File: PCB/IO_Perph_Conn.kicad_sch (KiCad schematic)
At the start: 7 parts, among them U2 STM32MP157FABx

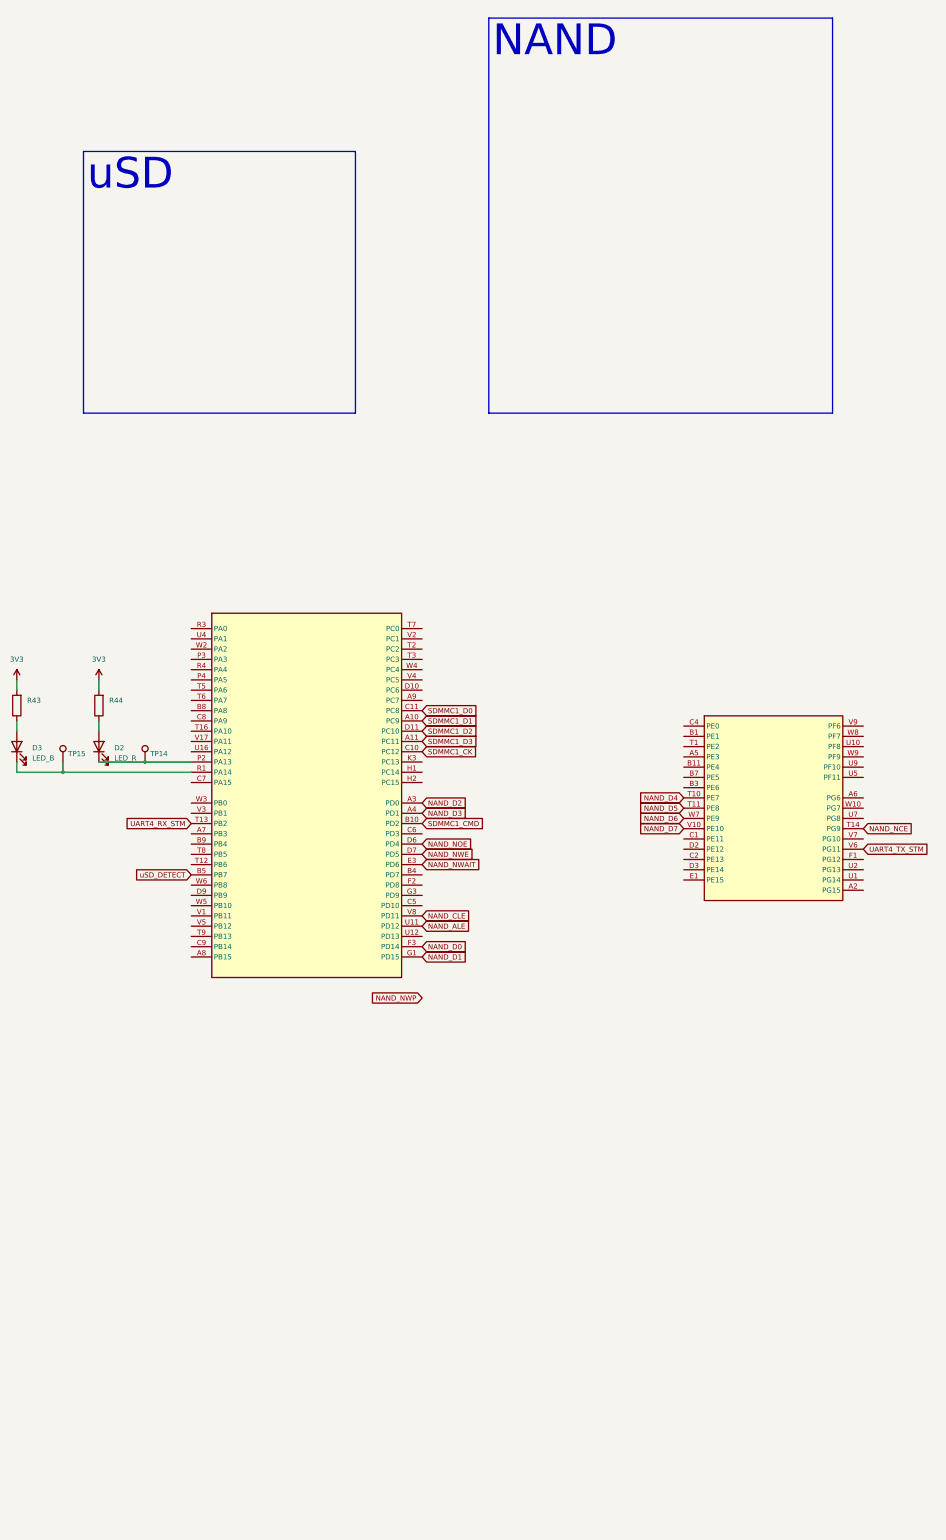
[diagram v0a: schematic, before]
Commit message: PCB_UPDATE
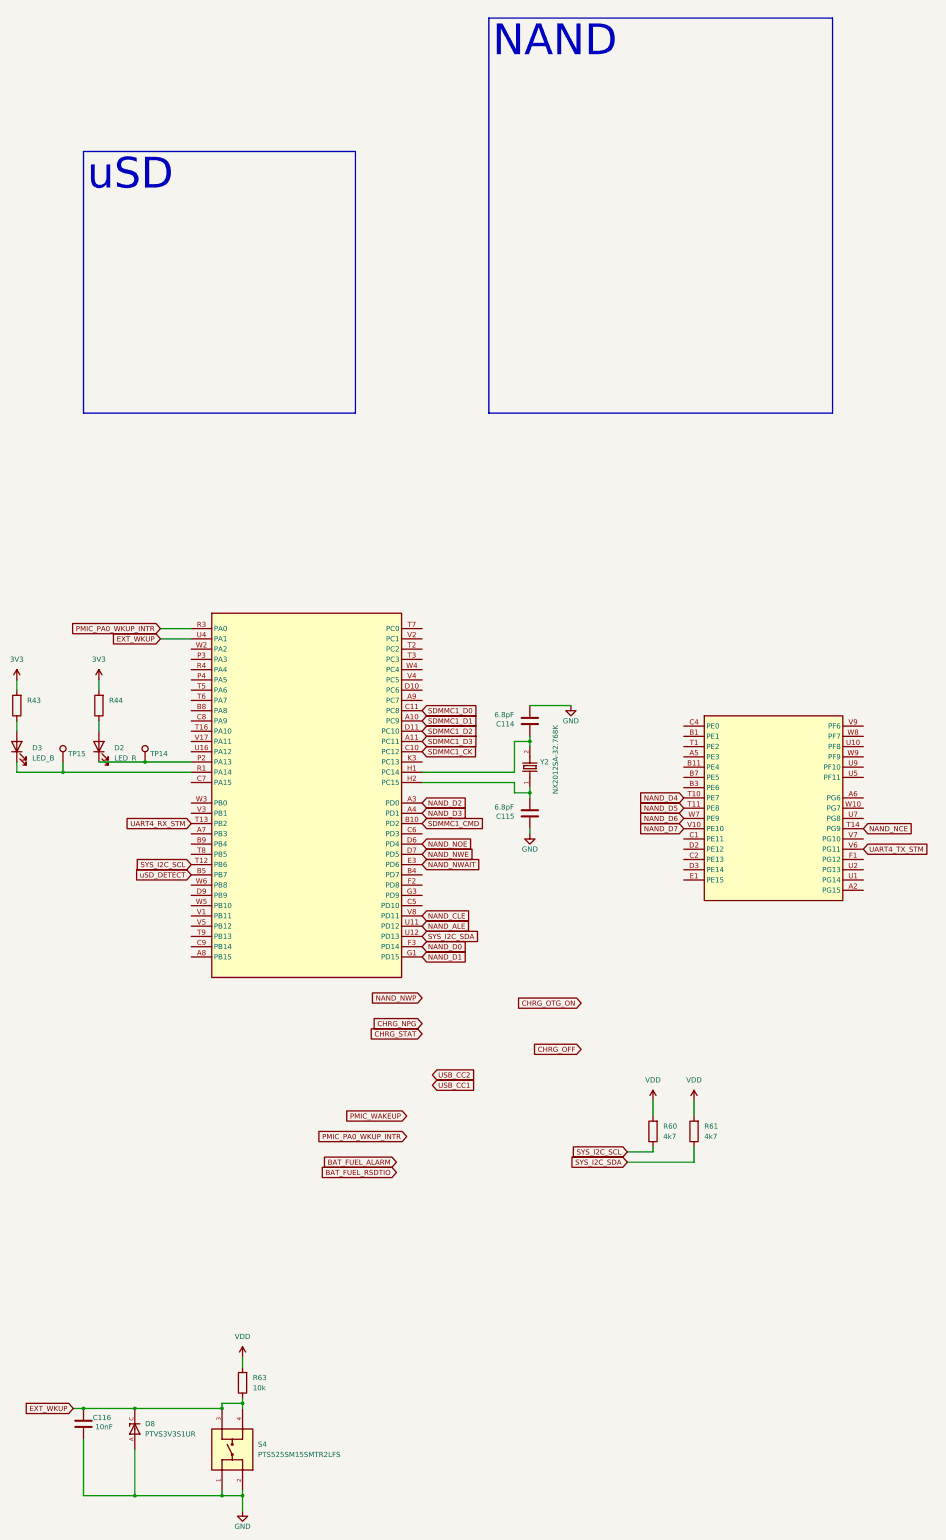
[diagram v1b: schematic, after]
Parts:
- added C114, C115: 6.8pF, Capacitor_SMD:C_0402_1005Metric, symbol Device:C
- added C116: 10nF, Capacitor_SMD:C_0402_1005Metric, symbol Device:C
- added D8: PTVS3V3S1UR, PTVS3V3S1UR:TVS_PTVS3V3S1UR, symbol PTVS3V3S1UR:PTVS3V3S1UR
- added R60, R61: 4k7, Resistor_SMD:R_0402_1005Metric, symbol Device:R
- added R63: 10k, Resistor_SMD:R_0402_1005Metric, symbol Device:R
- added S4: PTS525SM15SMTR2LFS, lib:SW_PTS525SM15SMTR2LFS, symbol PTS525SM15SMTR2LFS:PTS525SM15SMTR2LFS
- added Y2: NX2012SA-32.768K, lib:XTAL_NX2012SA-32.768K-STD-MUB-1, symbol NX2012SA-32.768K-STD-MUB-1:NX2012SA-32.768K-STD-MUB-1
- R43, R44: footprint (none) -> Resistor_SMD:R_0402_1005Metric
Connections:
- net at U2.H1 (PC14): now also C114.2, Y2.2
- net at U2.H2 (PC15): now also C115.1, Y2.1
- net PMIC_PA0_WKUP_INTR: now reaches U2.R3 (PA0)
- net SYS_I2C_SCL: now reaches U2.T12 (PB6)
- net SYS_I2C_SCL: now also R60.1
- net SYS_I2C_SDA: now reaches U2.U12 (PD13)
- net SYS_I2C_SDA: now also R61.1
- net EXT_WKUP: now reaches U2.U4 (PA1)
- net EXT_WKUP: now also C116.2, D8.C, R63.1, S4.3, S4.4
- new net GND: C114.1, C115.2, C116.1, D8.A, S4.1, S4.2
- new net VDD: R60.2, R61.2, R63.2
